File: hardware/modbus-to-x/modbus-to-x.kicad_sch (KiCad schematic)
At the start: 50 parts, among them J1 PWR, J2 UART, SW1 SW_Push, SW2 SW_Push, U1 AMS1117-3.3, U3 MAX3485, U4 ESP32-WROOM-32D, U5 AT24CS64-XHM, U6 AT24CS64-XHM, U7 LMR14020SQDPRTQ1

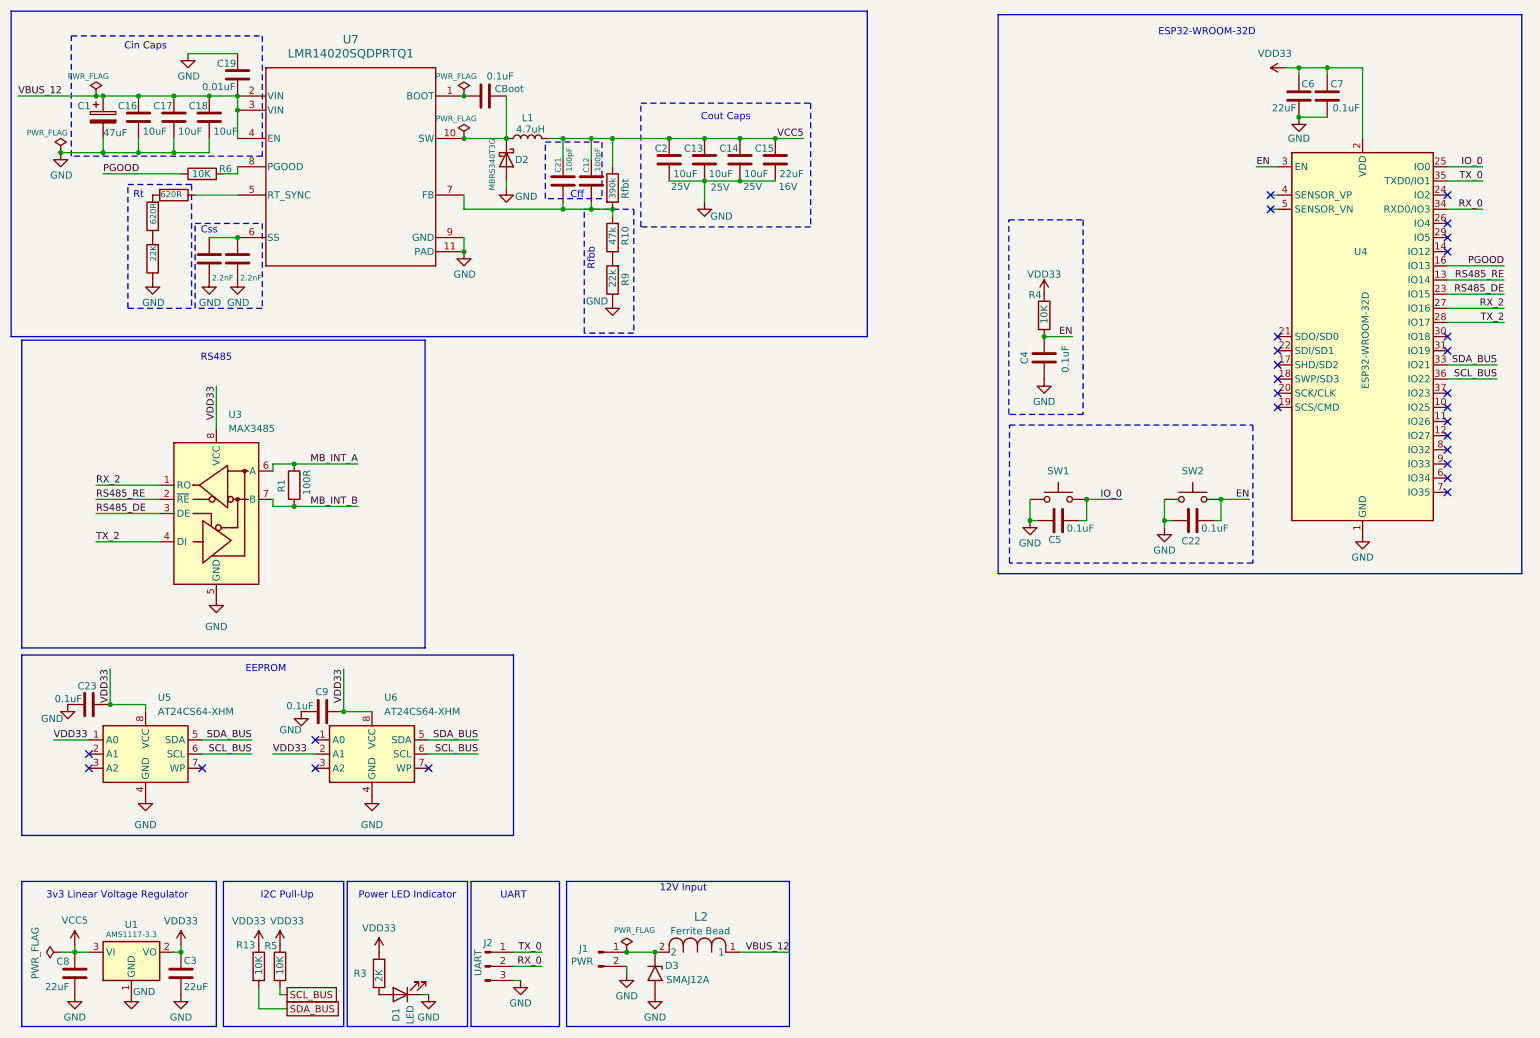
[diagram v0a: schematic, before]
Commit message: hardware tweaks
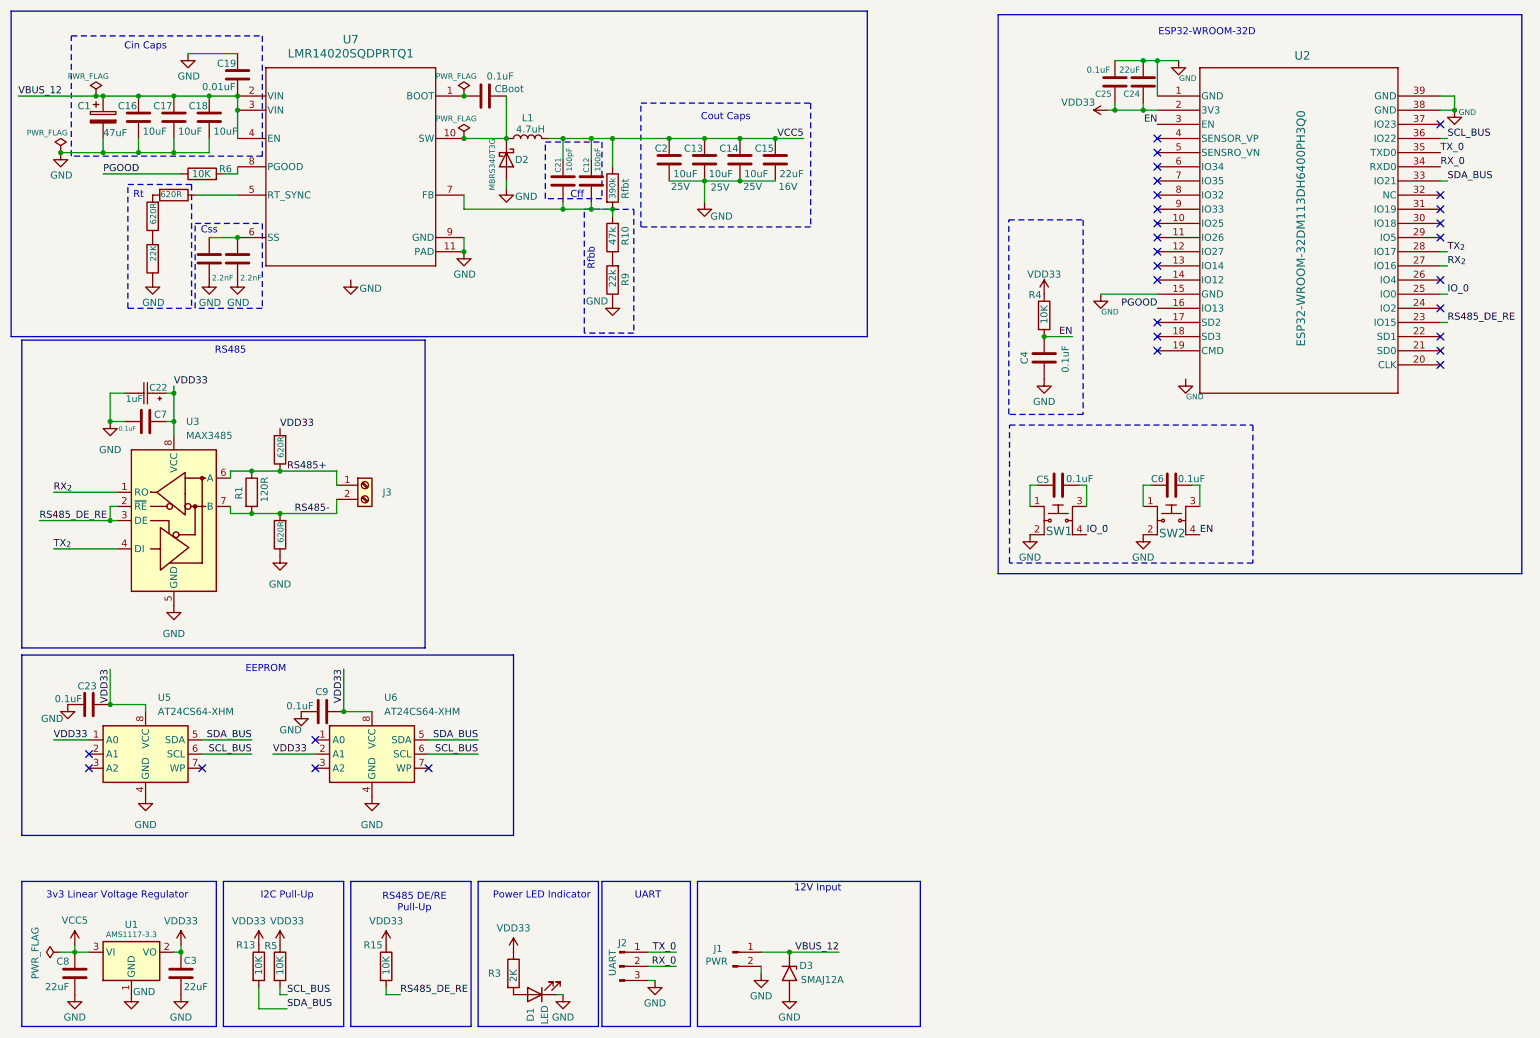
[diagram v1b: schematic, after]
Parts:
- removed C22: 0.1uF, Capacitor_SMD:C_1206_3216Metric_Pad1.33x1.80mm_HandSolder, symbol Device:C
- removed L2: MPZ1005S121CT000, MPZ1005S121CT000:IND_1005_TDK-L, symbol MPZ1005S121CT000:MPZ1005S121CT000
- removed SW1, SW2: SW_Push, Button_Switch_SMD:SW_SPST_Omron_B3FS-105xP, symbol Switch:SW_Push
- removed U4: ESP32-WROOM-32D, RF_Module:ESP32-WROOM-32D, symbol RF_Module:ESP32-WROOM-32D
- added C22: 1uF, CAP_UMA_3X5_NCH, symbol Nichicon 1uF Radial THT UMA1H010MCD2TP:UMA1H010MCD2TP
- added C24: 22uF, Capacitor_SMD:C_0805_2012Metric_Pad1.18x1.45mm_HandSolder, symbol Device:C
- added C25: 0.1uF, Capacitor_SMD:C_1206_3216Metric_Pad1.33x1.80mm_HandSolder, symbol Device:C
- added J3: Screw_Terminal_3.5mm_2, SparkFun-Connector:Screw_Terminal_3.5mm-2, symbol SparkFun-Connector:Screw_Terminal_3.5mm_2
- added R14, R2: 620R, Resistor_SMD:R_0805_2012Metric_Pad1.20x1.40mm_HandSolder, symbol Device:R
- added R15: 10K, Resistor_SMD:R_0805_2012Metric_Pad1.20x1.40mm_HandSolder, symbol Device:R
- added SW1, SW2: 1825910-7, digikey-footprints:Switch_Tactile_SMD_6x6mm_PTS645, symbol dk_Tactile-Switches:1825910-7
- added U2: ESP32-WROOM-32DM113DH6400PH3Q0, ESP32-WROOM-32D-M113DH6400PH3Q0:ESP32-WROOM-32DM113DH6400PH3Q0_EXP, symbol ESP32-WROOM-32D-M113DH6400PH3Q0:ESP32-WROOM-32DM113DH6400PH3Q0
- C6: value 22uF -> 0.1uF; footprint Capacitor_SMD:C_0805_2012Metric_Pad1.18x1.45mm_HandSolder -> Capacitor_SMD:C_1206_3216Metric_Pad1.33x1.80mm_HandSolder; PartNo CL21A226MOCLRNC -> CVNF100K12X; Voltage 16V -> 50V
- R1: value 100R -> 120R
- U7: footprint LMR14020SQDPRTQ1:DPR0010A -> LMR14020SQDPRTQ1:DPR0010A_3mm_thermals
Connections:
- net RS485_RE is gone; now on net RS485_DE_RE: U3.2 (~{RE})
- net EN: now also SW2.4, U2.3 (EN)
- net GND: now also C7.2, U7.V (GND_STITCH), C22.2, C24.1, C25.1, R14.1, SW1.2, SW2.2, U2.1 (GND), U2.15 (GND), U2.38 (GND), U2.39 (GND), U2.V (GND_STITCH); no longer C5.2, C6.1, C7.1
- net IO_0: now also SW1.4, U2.25 (IO0); no longer C5.1
- net PGOOD: now also U2.16 (IO13)
- net RX_0: now also U2.34 (RXD0)
- net SCL_BUS: now also U2.36 (IO22)
- net SDA_BUS: now also U2.33 (IO21)
- net TX_0: now also U2.35 (TXD0)
- net VBUS_12: now also D3.1 (A1), J1.1 (Pin_1)
- net VDD33: now also C7.1, C22.1, C24.2, C25.2, R15.1, R2.2, U2.2 (3V3); no longer C6.2, C7.2
- net MB_INT_A renamed RS485+
- net RS485+: now also J3.1 (Pin_1), R2.1
- net MB_INT_B renamed RS485-
- net RS485-: now also J3.2 (Pin_2), R14.2
- net RS485_DE renamed RS485_DE_RE
- net RS485_DE_RE: now also R15.2, U2.23 (IO15)
- net RX_2 renamed RX_{2}
- net RX_{2}: now also U2.27 (IO16)
- net TX_2 renamed TX_{2}
- net TX_{2}: now also U2.28 (IO17)
- new net: C5.2, SW1.1
- new net: C5.1, SW1.3
- new net: C6.1, SW2.3
- new net: C6.2, SW2.1
- no-connect marks 28 -> 30
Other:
- note added: "RS485 DE/RE Pull-Up"
- moved on the sheet: D1, D3, J1, J2, R1, R3, U3
